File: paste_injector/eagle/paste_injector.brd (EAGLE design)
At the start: 40 x 30 mm, 17 parts, among them IC1 ULN2003AD, J2 USB, J5 PINHD-2X3, Q2 CSTCR6M00G53Z, U4 ATMEGA328TQFP32

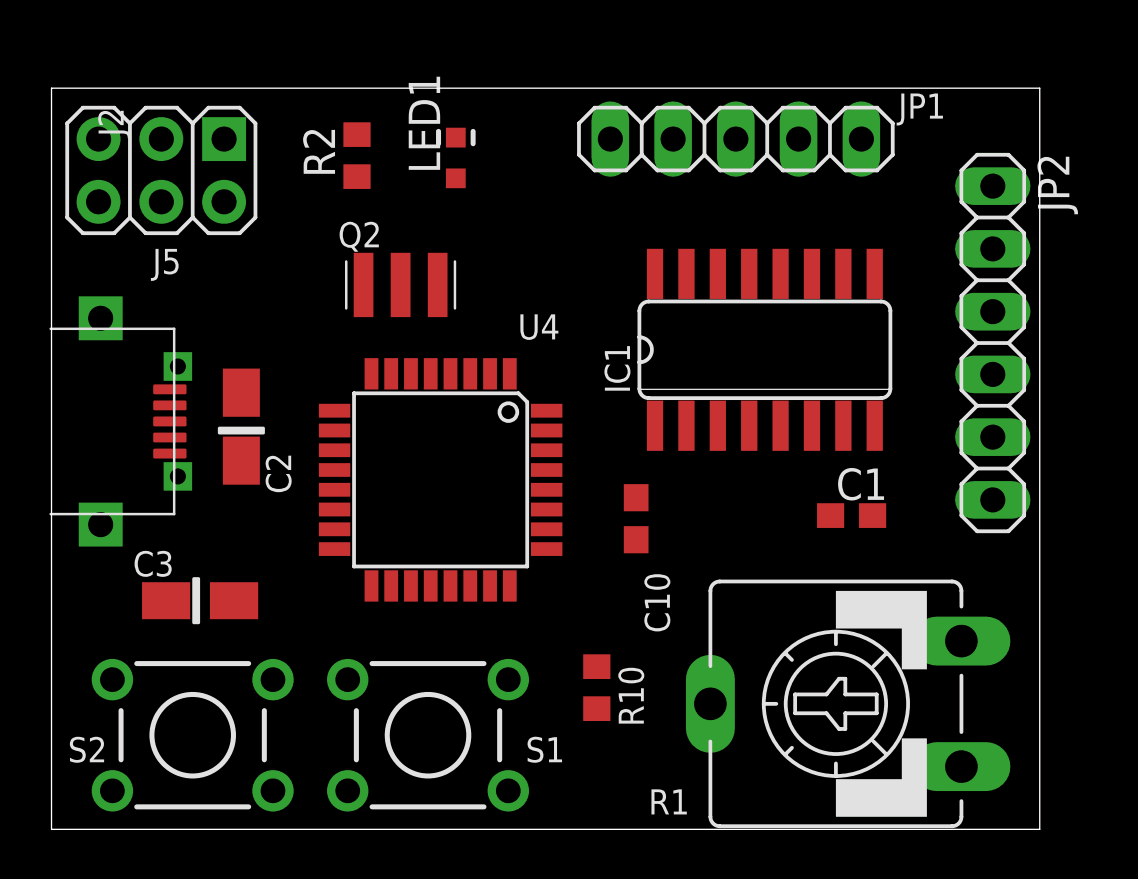
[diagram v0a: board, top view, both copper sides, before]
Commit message: Minor tweaks.
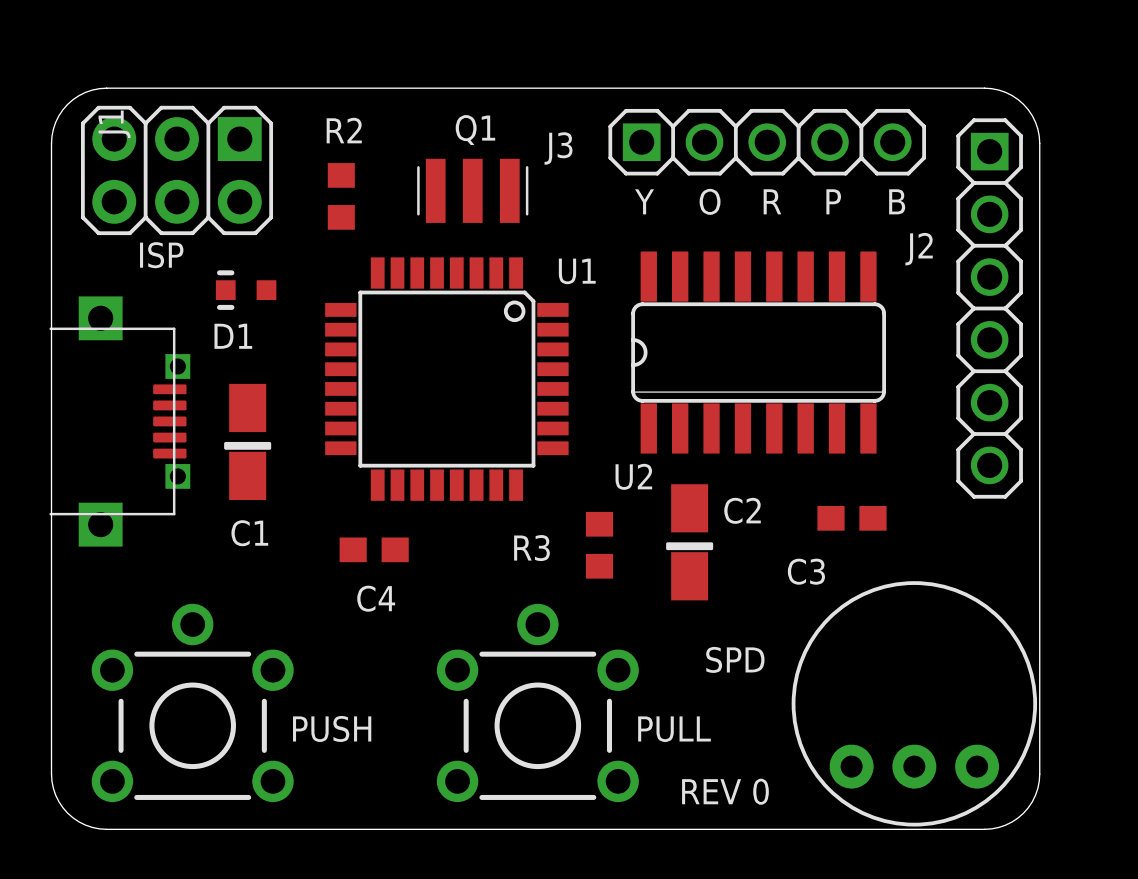
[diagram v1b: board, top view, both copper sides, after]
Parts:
- removed C10: 0.1uF, paste_injector:C0603
- removed IC1: ULN2003AD, paste_injector:SO16
- removed J5: PINHD-2X3, paste_injector:2X03
- removed JP1: (no value), paste_injector:1X05
- removed JP2: (no value), paste_injector:1X06
- removed LED1: (no value), arm-pro-mini-tester:LED0603
- removed Q2: CSTCR6M00G53Z, paste_injector:CSTCR6M
- removed R10: 5K, paste_injector:R0603
- removed U4: ATMEGA328TQFP32, paste_injector:TQFP32-08
- added C4: 0.1uF, paste_injector:C0603
- added D1: (no value), paste_injector:LED0603
- added ISP: PINHD-2X3, paste_injector:2X03
- added J1: USB, paste_injector:USB-MICRO-ZX62RD-AB-5P8
- added J3: (no value), paste_injector:1X05
- added Q1: CSTCR6M00G53Z, paste_injector:CSTCR6M
- added R3: 5K, paste_injector:R0603
- added U1: ATMEGA328TQFP32, paste_injector:TQFP32-08
- added U2: ULN2003AD, paste_injector:SO16
- C1: value 0.1uF -> 10uF; device paste_injector:C0603 -> paste_injector:A/3216-18R
- C3: value 10uF -> 0.1uF; device paste_injector:A/3216-18R -> paste_injector:C0603
- J2: value USB -> (none); device paste_injector:USB-MICRO-ZX62RD-AB-5P8 -> paste_injector:1X06
- R1: value (none) -> 10K; device paste_injector:CA9V -> paste_injector:TRIMPOT
- S1, S2: device paste_injector:TLE1105 -> paste_injector:PUSH_BUTTON
- moved J2 38.9 mm to (38.0, 21.1)
- moved C3 26.6 mm to (32.4, 12.6), turned to 0 degrees
- moved C1 24.6 mm to (7.94, 15.7), turned to 270 degrees
- moved C2 18.7 mm to (25.8, 11.6)
- moved S2 14.0 mm to (19.7, 4.19)
- moved S1 9.53 mm to (5.71, 4.19)
- moved R1 3.17 mm to (34.9, 5.08), turned to 0 degrees
- moved R2 1.77 mm to (11.7, 25.6)
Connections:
- net +5V: now also C1.+, C4.1, ISP.2, J1.1, J2.3, J3.3, R1.CW, R3.2, U1.18, U1.4, U1.6, U2.9; no longer C10.1, C3.+, IC1.9, J2.1, J5.2, JP1.3, JP2.3, R1.E, R10.2, U4.18, U4.4, U4.6
- net BACKWARD: now also S2.B1, U1.11; no longer S1.B, U4.11
- net DTR: now also C3.2, J2.6; no longer C1.2, JP2.6
- net FORWARD: now also S1.B1, U1.10; no longer S2.B, U4.10
- net GND: now also C1.-, C4.2, D1.C, ISP.6, J1.5, J2.1, J2.2, Q1.2, R1.CCW, S1.A1, S1.GND, S2.A1, S2.GND, U1.21, U1.3, U1.5, U2.5, U2.6, U2.7, U2.8; no longer C10.2, C3.-, IC1.5, IC1.6, IC1.7, IC1.8, J2.5, J5.6, JP2.1, JP2.2, LED1.C, Q2.2, R1.A, S1.A, S2.A, U4.21, U4.3, U4.5
- net M1: now also U1.32, U2.1; no longer IC1.1, U4.25
- net M1-BLUE: now also J3.5, U2.16; no longer IC1.16, JP1.5
- net M2: now also U1.1, U2.2; no longer IC1.2, U4.26
- net M2-PINK: now also J3.4, U2.15; no longer IC1.15, JP1.4
- net M3: now also U1.2, U2.3; no longer IC1.3, U4.19
- net M3-YELOW: now also J3.1, U2.14; no longer IC1.14, JP1.1
- net M4: now also U1.9, U2.4; no longer IC1.4, U4.22
- net M4-ORANGE: now also J3.2, U2.13; no longer IC1.13, JP1.2
- net MISO: now also ISP.1, U1.16; no longer J5.1, U4.16
- net MOSI: now also ISP.4, U1.15; no longer J5.4, U4.15
- net N$1: now also D1.A; no longer LED1.A
- net N$2: now also Q1.1, U1.7; no longer Q2.1, U4.7
- net N$7: now also Q1.3, U1.8; no longer Q2.3, U4.8
- net POT: now also R1.C, U1.23; no longer R1.S, U4.23
- net RESET: now also C3.1, ISP.5, R3.1, U1.29; no longer C1.1, J5.5, R10.1, U4.29
- net RXI: now also J2.4, U1.30; no longer JP2.4, U4.30
- net SCK/LED: now also ISP.3, U1.17; no longer J5.3, U4.17
- net TXO: now also J2.5, U1.31; no longer JP2.5, U4.31
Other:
- outline, holes or cut-outs redrawn
- board text added: "B"
- board text added: "O"
- board text added: "P"
- board text added: "PULL"
- board text added: "PUSH"
- board text added: "R"
- board text added: "REV 0"
- board text added: "SPD"
- board text added: "Y"
